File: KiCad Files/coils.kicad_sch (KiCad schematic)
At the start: 14 parts, among them Q1 AO3400A, Q2 AO3400A, Q3 AO3400A, Q4 AO3400A, Q5 AO3401A, Q6 AO3401A, Q7 AO3401A, Q8 AO3401A, U1 74HC595

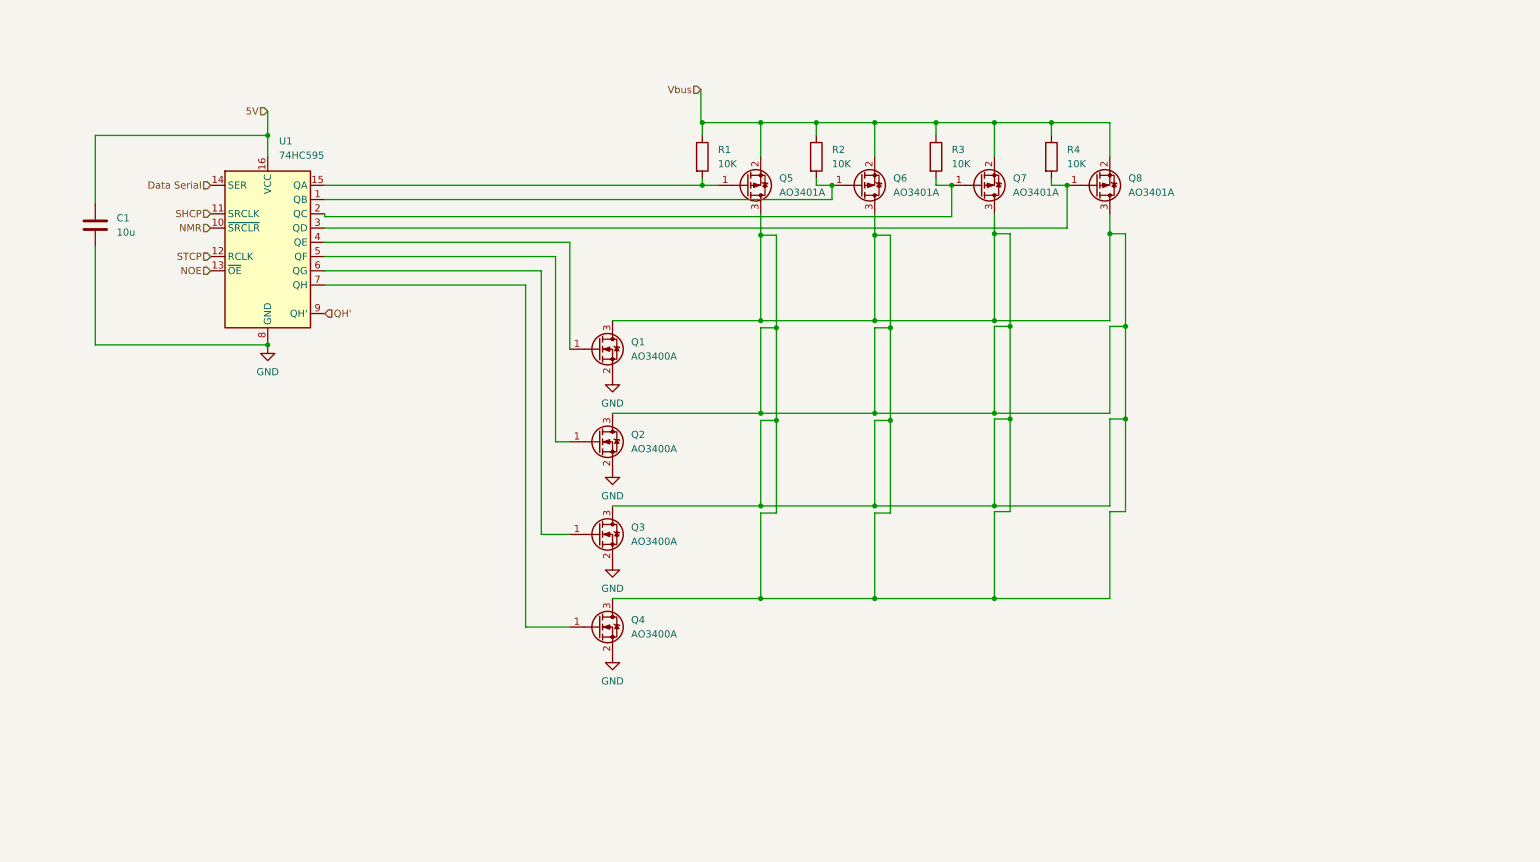
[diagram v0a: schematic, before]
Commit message: Mosfet crazy town
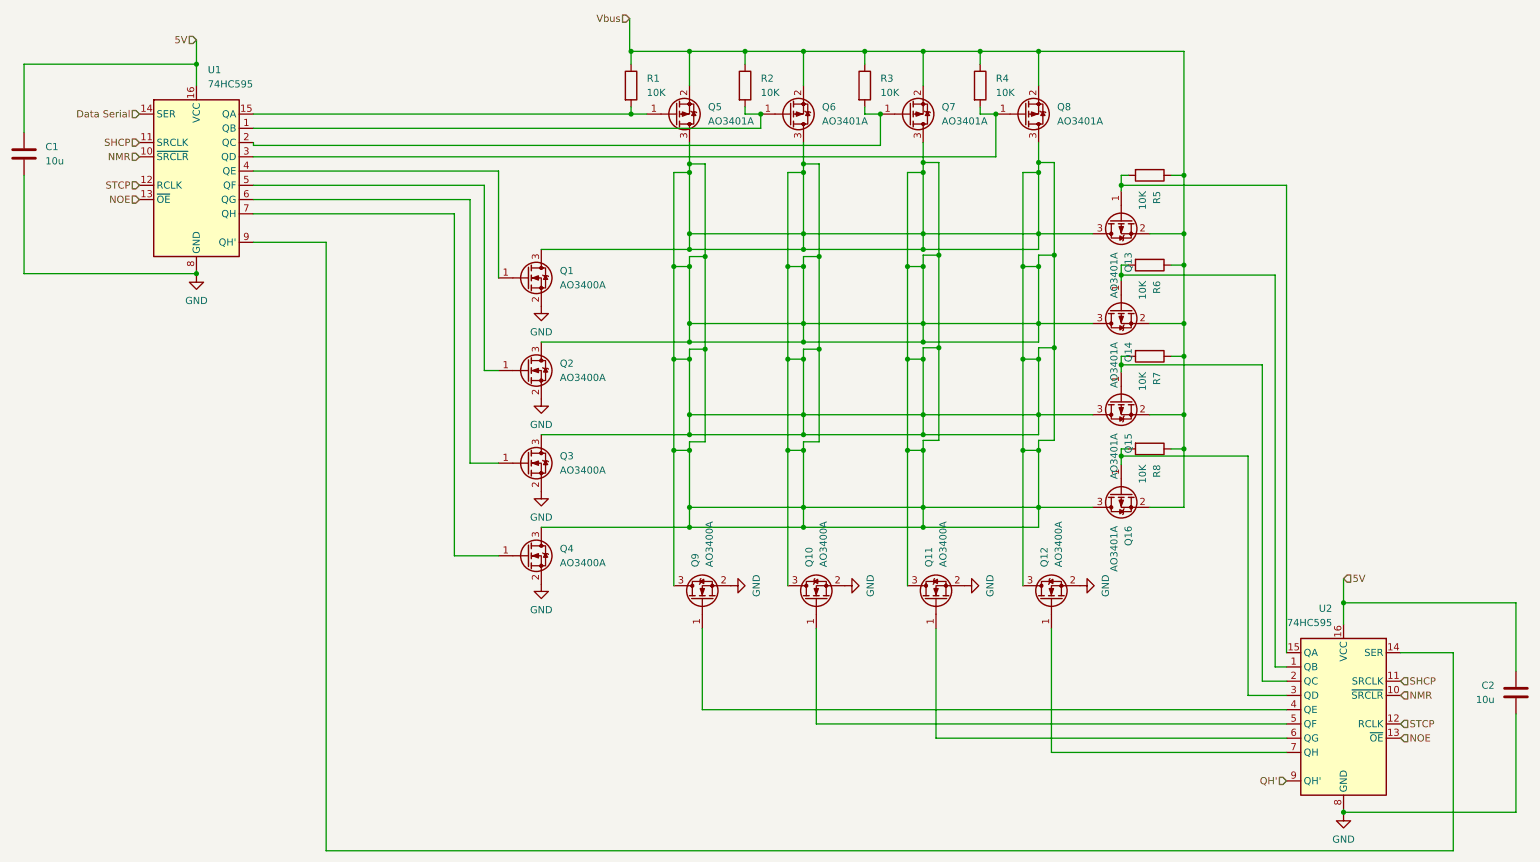
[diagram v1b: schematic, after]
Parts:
- added C2: 10u, Capacitor_SMD:C_0805_2012Metric, symbol Device:C
- added Q10, Q11, Q12, Q9: AO3400A, Package_TO_SOT_SMD:SOT-23, symbol Transistor_FET:AO3400A
- added Q13, Q14, Q15, Q16: AO3401A, Package_TO_SOT_SMD:SOT-23, symbol Transistor_FET:AO3401A
- added R5, R6, R7, R8: 10K, Resistor_SMD:R_0603_1608Metric, symbol Device:R
- added U2: 74HC595, 74HC595:SO16, symbol 74xx:74HC595
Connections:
- net 5V: now also C2.1, U2.16 (VCC)
- net GND: now also C2.2, Q10.2 (S), Q11.2 (S), Q12.2 (S), Q9.2 (S), U2.8 (GND)
- net NMR: now also U2.10 (~{SRCLR})
- net NOE: now also U2.13 (~{OE})
- net QH': now also U2.9 (QH'); no longer U1.9 (QH')
- net SHCP: now also U2.11 (SRCLK)
- net STCP: now also U2.12 (RCLK)
- net Vbus: now also Q13.2 (S), Q14.2 (S), Q15.2 (S), Q16.2 (S), R5.1, R6.1, R7.1, R8.1
- net at Q1.3 (D), Q2.3 (D), Q3.3 (D)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: now also Q10.3 (D), Q11.3 (D), Q12.3 (D), Q13.3 (D), Q14.3 (D), Q15.3 (D), Q16.3 (D), Q9.3 (D)
- new net: Q14.1 (G), R6.2, U2.1 (QB)
- new net: Q16.1 (G), R8.2, U2.3 (QD)
- new net: Q13.1 (G), R5.2, U2.15 (QA)
- new net: U1.9 (QH'), U2.14 (SER)
- new net: Q15.1 (G), R7.2, U2.2 (QC)
- new net: Q9.1 (G), U2.4 (QE)
- new net: Q10.1 (G), U2.5 (QF)
- new net: Q11.1 (G), U2.6 (QG)
- new net: Q12.1 (G), U2.7 (QH)
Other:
- moved on the sheet: C1, Q1, Q2, Q3, Q4, Q5, Q6, Q7, Q8, R1, R2, R3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
